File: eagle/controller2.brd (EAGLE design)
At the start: 77.1 x 48.2 mm, 18 parts, among them K1 SRD-05VDC-SL-C, K2 SRD-05VDC-SL-C, T1 BC547, T2 BC547, X1 VCC, X2 IN1, X3 IN2

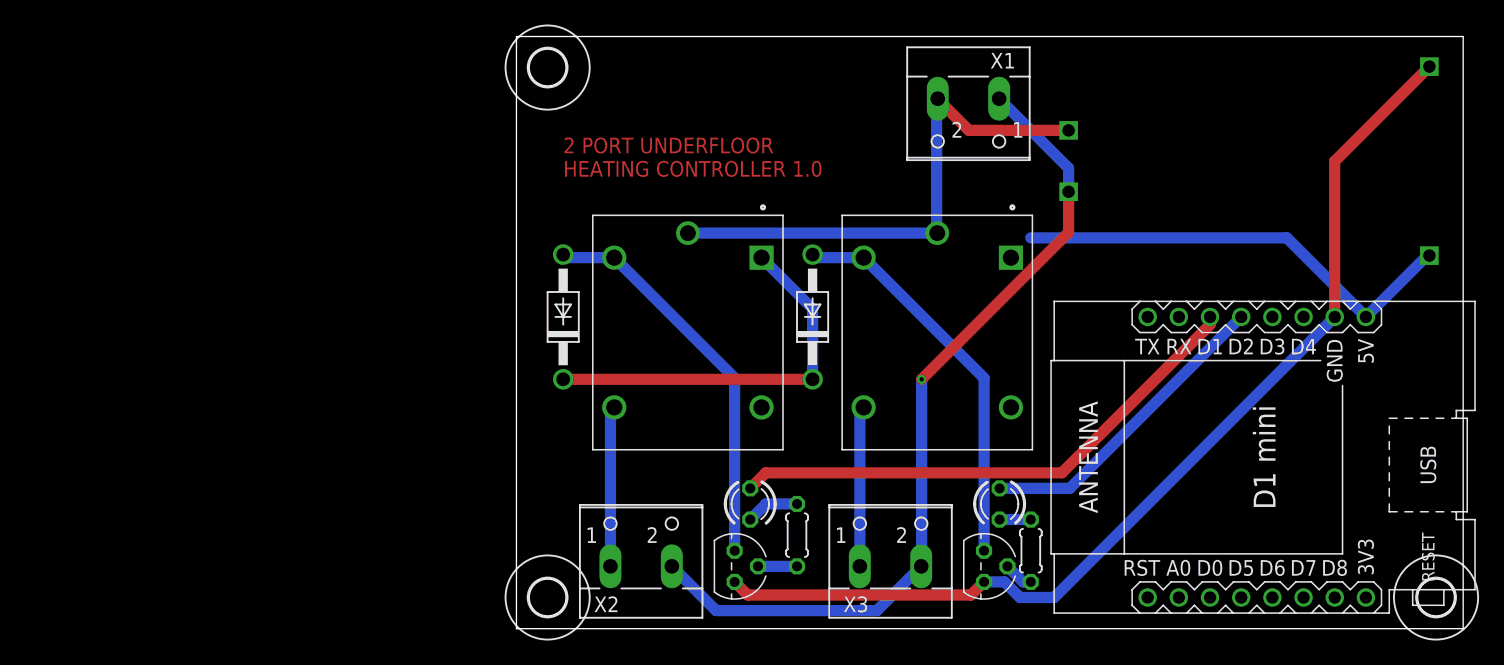
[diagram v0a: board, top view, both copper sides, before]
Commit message: Update to Version 1.1
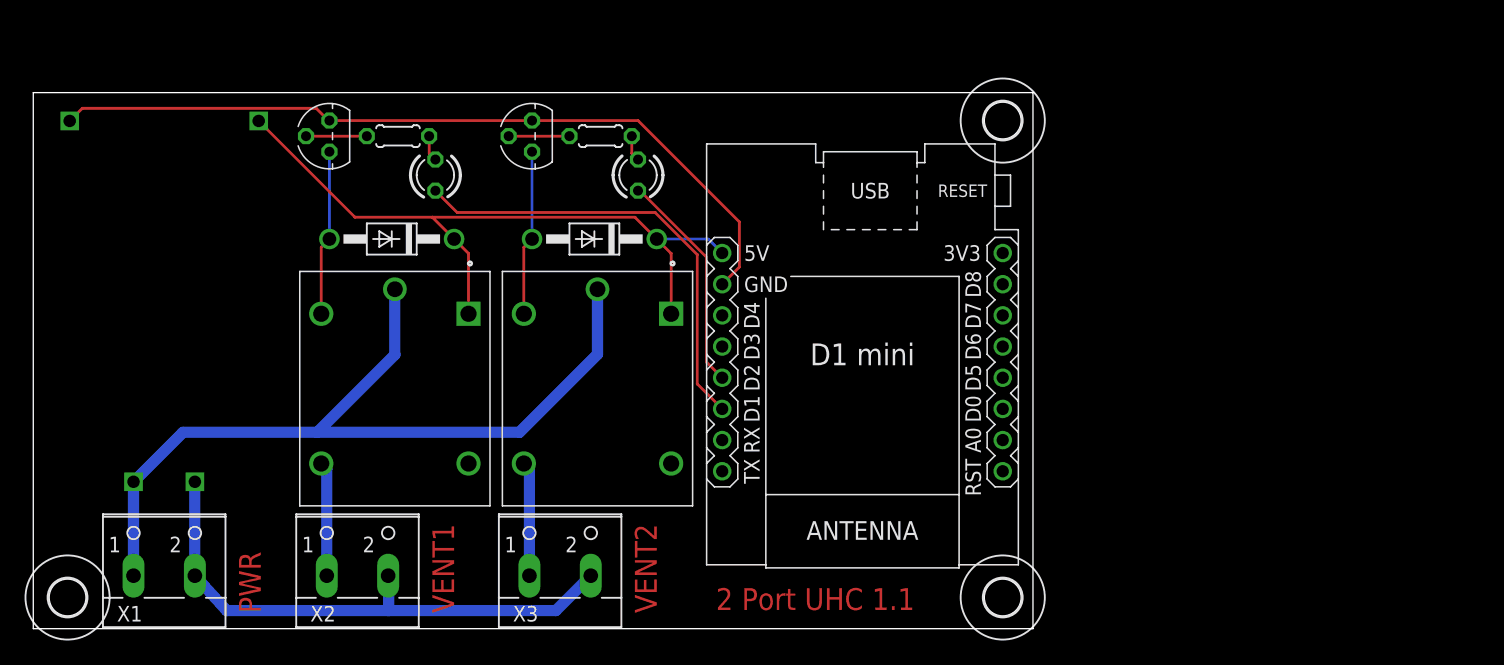
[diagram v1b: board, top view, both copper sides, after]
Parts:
- moved HLK1 89.1 mm to (10.7, 26.7), turned to 90 degrees
- moved X1 74.9 mm to (10.7, 5.59), turned to 0 degrees
- moved U$2 56.9 mm to (79.0, 2.54)
- moved U$4 52.5 mm to (79.0, 41.4)
- moved T2 50.8 mm to (40.6, 40.1), turned to 90 degrees
- moved R2 48.7 mm to (46.2, 40.1), turned to 180 degrees
- moved T1 48.2 mm to (24.1, 40.1), turned to 90 degrees
- moved R1 46.0 mm to (29.7, 40.1), turned to 180 degrees
- moved LED2 39.8 mm to (49.3, 37.0), turned to 90 degrees
- moved U$3 39.1 mm to (2.79, 2.54)
- moved LED1 37.1 mm to (32.8, 37.0), turned to 90 degrees
- moved U$1 33.8 mm to (67.6, 22.4), turned to 180 degrees
- moved K2 28.1 mm to (46.0, 19.6)
- moved X3 26.9 mm to (42.9, 5.59)
- moved K1 24.3 mm to (29.5, 19.6)
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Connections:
- net 0V: now also X1.2; no longer X1.1
- net VCC: now also X1.1; no longer X1.2
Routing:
- net VCC: track 43.0 -> 69.3 mm
- net 0V: track 69.0 -> 45.4 mm, vias 1 -> 0
- net GND: track 83.4 -> 64.5 mm
- net N$3: track 32.2 -> 13.5 mm
- net N$1: track 32.2 -> 13.6 mm
- net +5V: track 69.3 -> 57.9 mm
- net N$14: track 25.5 -> 18.2 mm
- net N$15: track 43.6 -> 36.9 mm
- net N$2: track 13.1 -> 9.33 mm
- net N$11: track 13.1 -> 9.33 mm
- net N$8: track 2.43 -> 4.95 mm
- net N$20: track 4.34 -> 2.12 mm
- net N$9: track 3.17 -> 4.95 mm
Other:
- board size 77.1 x 48.2 mm -> 81.5 x 43.7 mm
- board text added: "2 Port UHC 1.1"
- board text added: "PWR"
- board text added: "VENT1"
- board text added: "VENT2"
- board text removed: "2 PORT UNDERFLOOR HEATING CONTROLLER 1.0"
